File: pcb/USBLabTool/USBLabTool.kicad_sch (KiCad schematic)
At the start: 0 parts

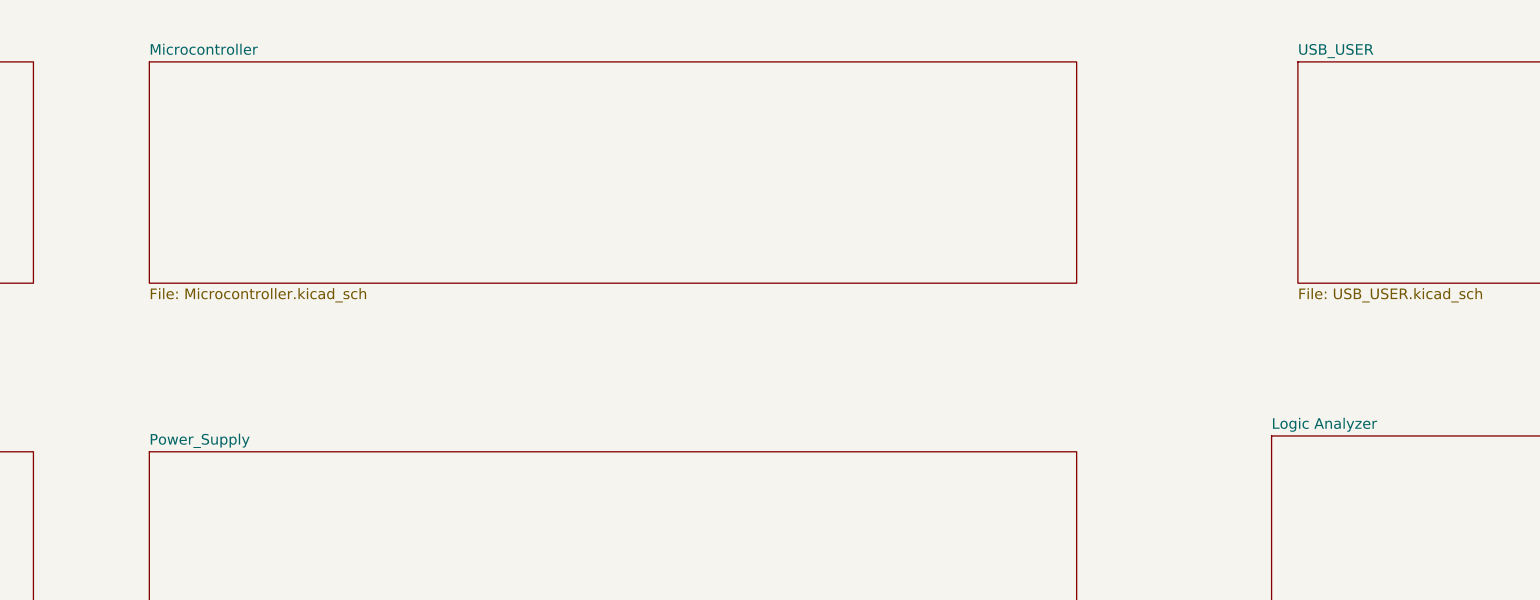
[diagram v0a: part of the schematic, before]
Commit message: merge from V2
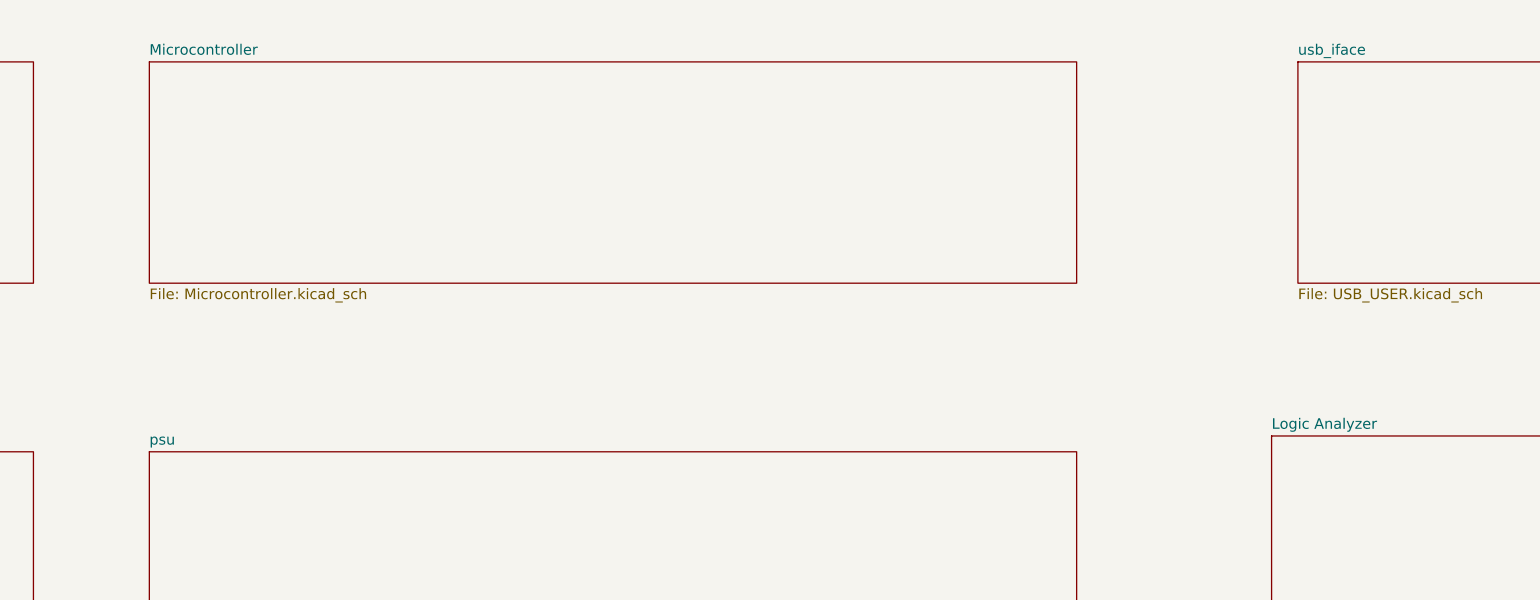
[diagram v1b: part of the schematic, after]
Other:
- sheet Power_Supply renamed psu
- sheet USB_USER renamed usb_iface
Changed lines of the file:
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@@
 			(color 0 0 0 0.0000)
 		)
-		(property "Sheetname" "USB_USER"
+		(property "Sheetname" "usb_iface"
 			(at 297.18 36.1184 0)
 			(effects
@@
 			(color 0 0 0 0.0000)
 		)
-		(property "Sheetname" "Power_Supply"
+		(property "Sheetname" "psu"
 			(at 158.75 83.1084 0)
 			(effects
